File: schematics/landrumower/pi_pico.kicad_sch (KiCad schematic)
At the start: 1 part, among them U1 Pico

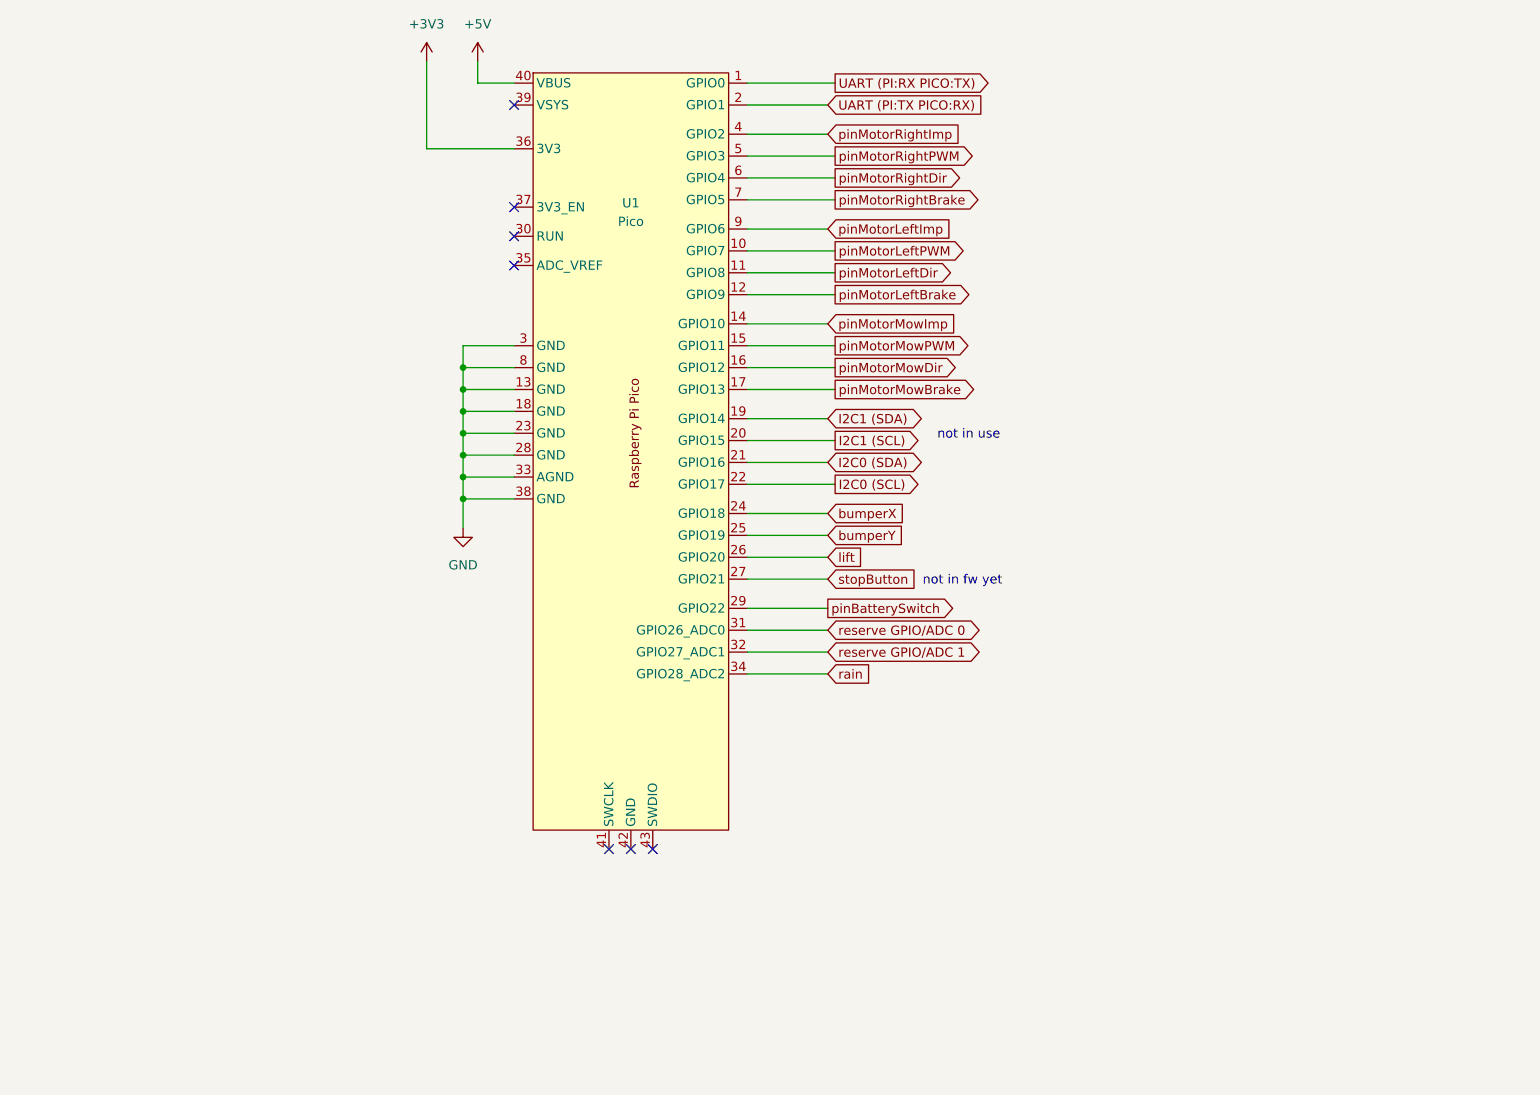
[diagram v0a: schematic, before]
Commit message: PCB changes for Landrumower
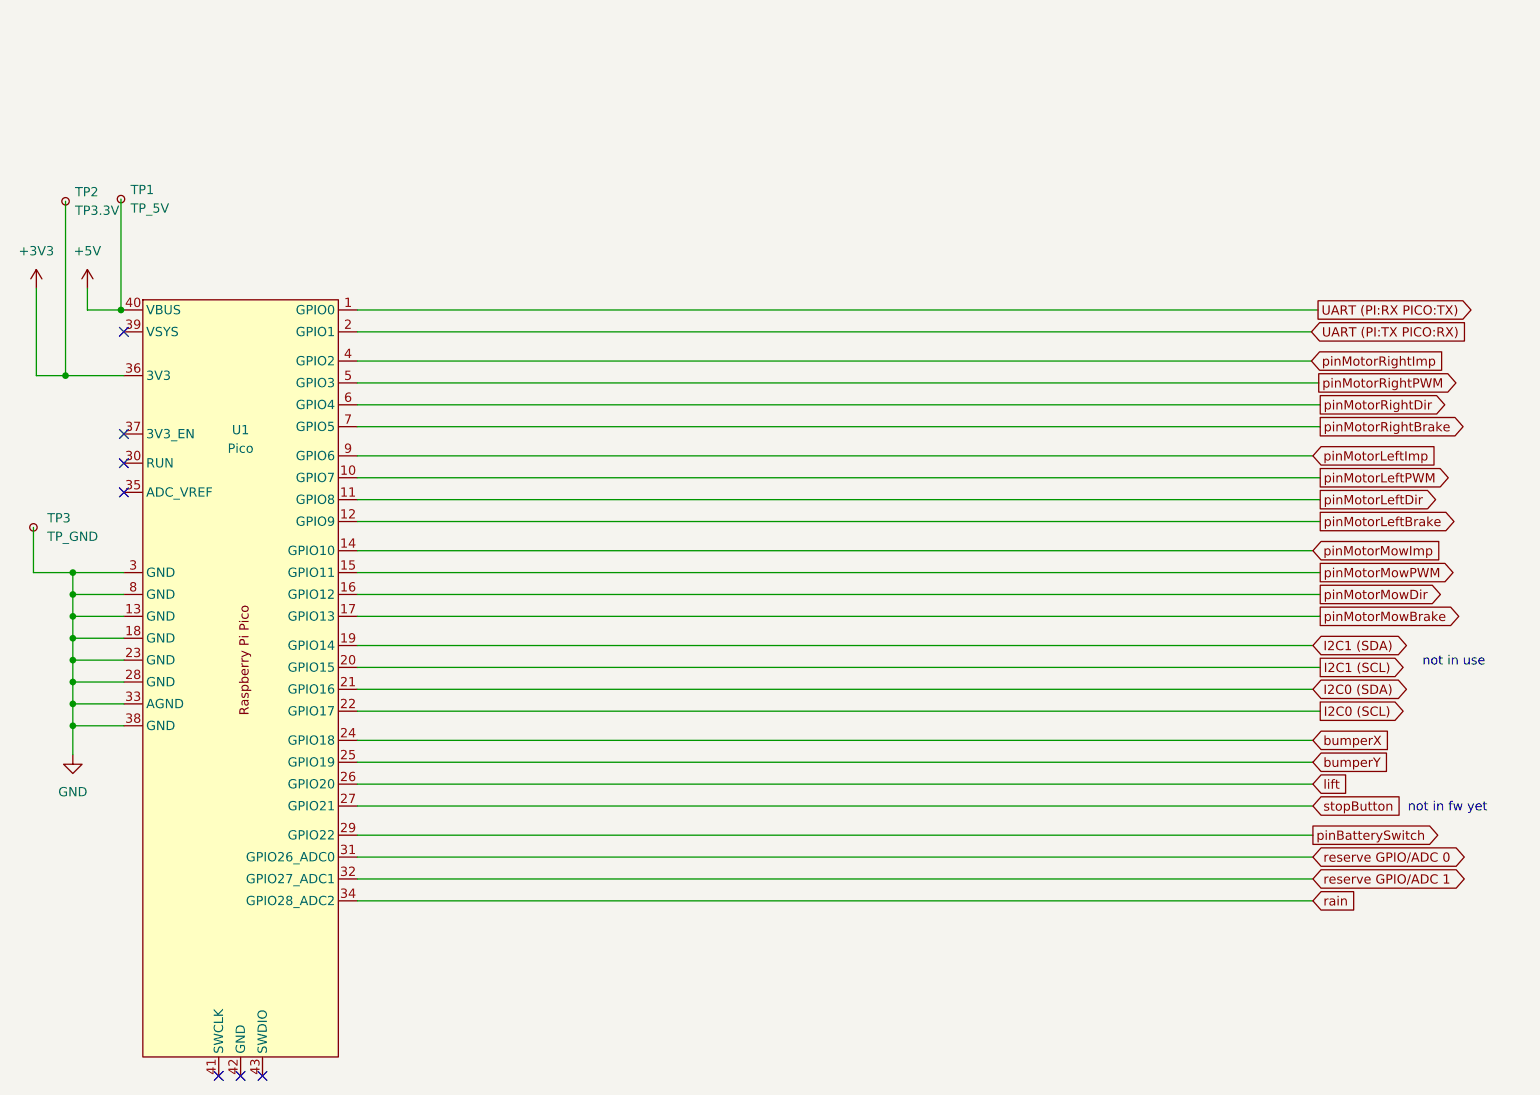
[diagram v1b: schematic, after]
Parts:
- added TP1: TP_5V, TestPoint:TestPoint_Pad_D2.0mm, symbol Connector:TestPoint_Small
- added TP2: TP3.3V, TestPoint:TestPoint_Pad_D2.0mm, symbol Connector:TestPoint_Small
- added TP3: TP_GND, TestPoint:TestPoint_Pad_D2.0mm, symbol Connector:TestPoint_Small
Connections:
- net +3V3: now also TP2.1
- net +5V: now also TP1.1
- net GND: now also TP3.1
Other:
- moved on the sheet: U1
